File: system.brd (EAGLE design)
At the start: 160 x 100 mm, 131 parts, among them IC1 TPS7B8650BQDDARQ1, IC2 TLV9101IDBVR, IC3 TLV9101IDBVR, J1 TSW-104-07-F-S, J2 163-179PH-EX, J3 RS1-02-G, SW1 1825910-6, SW2 1825910-6, SW3 1825910-6, U1 ATMEGA328PB-AU, Y1 ABL-16.000MHZ-B2

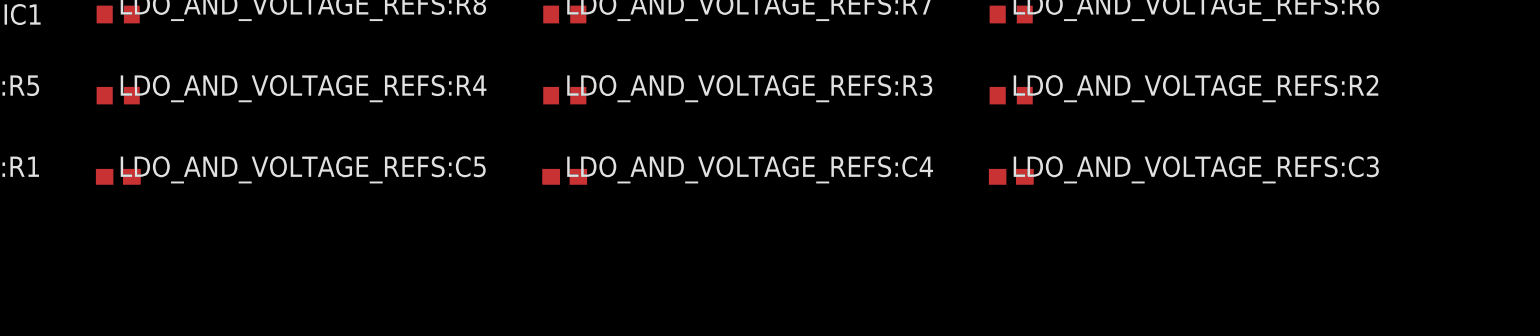
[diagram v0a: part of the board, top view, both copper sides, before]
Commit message: update some stuff
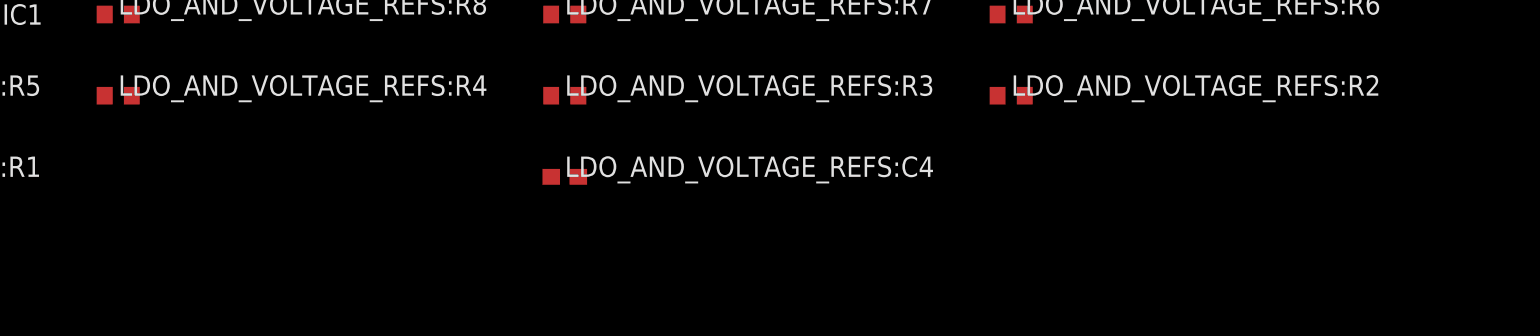
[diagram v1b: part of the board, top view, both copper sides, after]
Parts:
- removed LDO_AND_VOLTAGE_REFS:C3, LDO_AND_VOLTAGE_REFS:C5: 1uF, rcl:C0603
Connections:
- net 0: no longer LDO_AND_VOLTAGE_REFS:C3.2, LDO_AND_VOLTAGE_REFS:C5.2
- net VS_1.5V: no longer LDO_AND_VOLTAGE_REFS:C3.1
- net VS_2.5V: no longer LDO_AND_VOLTAGE_REFS:C5.1
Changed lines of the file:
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@@
 <attribute name="VALUE" x="-114.3" y="2.54" size="1.27" layer="27"/>
-</element>
-<element name="LDO_AND_VOLTAGE_REFS:C3" library="rcl" library_urn="urn:adsk.eagle:library:334" package="C0603" package3d_urn="urn:adsk.eagle:package:23616/2" value="1uF" x="-39.37" y="36.83" smashed="yes">
-<attribute name="NAME" x="-39.37" y="36.83" size="1.27" layer="25"/>
-<attribute name="POPULARITY" value="37" x="-39.37" y="36.83" size="1.778" layer="27" display="off"/>
-<attribute name="SPICEPREFIX" value="C" x="-39.37" y="36.83" size="1.778" layer="27" display="off"/>
-<attribute name="VALUE" x="-39.37" y="36.83" size="1.27" layer="27"/>
 </element>
 <element name="LDO_AND_VOLTAGE_REFS:C4" library="rcl" library_urn="urn:adsk.eagle:library:334" package="C0603" package3d_urn="urn:adsk.eagle:package:23616/2" value="1uF" x="-67.31" y="36.83" smashed="yes">
@@
 <attribute name="SPICEPREFIX" value="C" x="-67.31" y="36.83" size="1.778" layer="27" display="off"/>
 <attribute name="VALUE" x="-67.31" y="36.83" size="1.27" layer="27"/>
-</element>
-<element name="LDO_AND_VOLTAGE_REFS:C5" library="rcl" library_urn="urn:adsk.eagle:library:334" package="C0603" package3d_urn="urn:adsk.eagle:package:23616/2" value="1uF" x="-95.25" y="36.83" smashed="yes">
-<attribute name="NAME" x="-95.25" y="36.83" size="1.27" layer="25"/>
-<attribute name="POPULARITY" value="37" x="-95.25" y="36.83" size="1.778" layer="27" display="off"/>
-<attribute name="SPICEPREFIX" value="C" x="-95.25" y="36.83" size="1.778" layer="27" display="off"/>
-<attribute name="VALUE" x="-95.25" y="36.83" size="1.27" layer="27"/>
 </element>
 <element name="LDO_AND_VOLTAGE_REFS:IC1" library="TLV9101IDBVR" package="SOT95P280X145-5N" value="TLV9101IDBVR" x="-111.76" y="46.99" smashed="yes">
@@
 <contactref element="LDO_AND_VOLTAGE_REFS:IC3" pad="4"/>
 <contactref element="LDO_AND_VOLTAGE_REFS:IC3" pad="1"/>
-<contactref element="LDO_AND_VOLTAGE_REFS:C3" pad="1"/>
 <wire x1="-58.4" y1="53.02" x2="-104.99" y2="205.74" width="0" layer="19" extent="1-1"/>
 <wire x1="-55.9" y1="51.12" x2="-58.4" y2="53.02" width="0" layer="19" extent="1-1"/>
-<wire x1="-40.22" y1="36.83" x2="-55.9" y2="51.12" width="0" layer="19" extent="1-1"/>
 </signal>
 <signal name="VS_2.5V">
@@
 <contactref element="LDO_AND_VOLTAGE_REFS:IC2" pad="1"/>
 <contactref element="LDO_AND_VOLTAGE_REFS:IC2" pad="4"/>
-<contactref element="LDO_AND_VOLTAGE_REFS:C5" pad="1"/>
 <wire x1="-29.19" y1="53.02" x2="-49.11" y2="205.74" width="0" layer="19" extent="1-1"/>
 <wire x1="-26.69" y1="51.12" x2="-29.19" y2="53.02" width="0" layer="19" extent="1-1"/>
-<wire x1="-96.1" y1="36.83" x2="-29.19" y2="53.02" width="0" layer="19" extent="1-1"/>
 </signal>
 <signal name="ADC_EXT_INT">
@@
 <contactref element="BATTERY_AND_BUCK:C5" pad="2"/>
 <contactref element="BATTERY_AND_BUCK:C6" pad="2"/>
-<contactref element="LDO_AND_VOLTAGE_REFS:C5" pad="2"/>
 <contactref element="LDO_AND_VOLTAGE_REFS:IC3" pad="2"/>
 <contactref element="LDO_AND_VOLTAGE_REFS:IC1" pad="2"/>
@@
 <contactref element="LDO_AND_VOLTAGE_REFS:IC2" pad="2"/>
 <contactref element="LDO_AND_VOLTAGE_REFS:J1" pad="2"/>
-<contactref element="LDO_AND_VOLTAGE_REFS:C3" pad="2"/>
 <contactref element="LDO_AND_VOLTAGE_REFS:R6" pad="1"/>
 <contactref element="BANDGAP_REF:Q1" pad="5"/>
@@
 <wire x1="-40.22" y1="46.99" x2="-29.19" y2="52.07" width="0" layer="19" extent="1-1"/>
 <wire x1="-40.22" y1="41.91" x2="-40.22" y2="46.99" width="0" layer="19" extent="1-1"/>
-<wire x1="-38.52" y1="36.83" x2="-40.22" y2="41.91" width="0" layer="19" extent="1-1"/>
-<wire x1="-35.56" y1="20.32" x2="-38.52" y2="36.83" width="0" layer="19" extent="1-1"/>
 <wire x1="-58.4" y1="52.07" x2="-40.22" y2="46.99" width="0" layer="19" extent="1-1"/>
 <wire x1="-57.59" y1="68.18" x2="-58.4" y2="52.07" width="0" layer="19" extent="1-1"/>
 <wire x1="-49.09" y1="68.98" x2="-57.59" y2="68.18" width="0" layer="19" extent="1-1"/>
 <wire x1="-66.46" y1="36.83" x2="-58.4" y2="52.07" width="0" layer="19" extent="1-1"/>
+<wire x1="-35.56" y1="20.32" x2="-40.22" y2="41.91" width="0" layer="19" extent="1-1"/>
 <wire x1="-131.23" y1="102.87" x2="-107.1" y2="102.87" width="0" layer="19" extent="1-1"/>
 <wire x1="-132.93" y1="90.17" x2="-131.23" y2="102.87" width="0" layer="19" extent="1-1"/>
-<wire x1="-94.4" y1="36.83" x2="-66.46" y2="36.83" width="0" layer="19" extent="1-1"/>
-<wire x1="-96.1" y1="41.91" x2="-94.4" y2="36.83" width="0" layer="19" extent="1-1"/>
-<wire x1="-113.01" y1="46.99" x2="-96.1" y2="41.91" width="0" layer="19" extent="1-1"/>
 <wire x1="-99.48" y1="161.29" x2="-70.27" y2="161.29" width="0" layer="19" extent="1-1"/>
 <wire x1="-128.69" y1="161.29" x2="-99.48" y2="161.29" width="0" layer="19" extent="1-1"/>
-<wire x1="-85.51" y1="2.54" x2="-94.4" y2="36.83" width="0" layer="19" extent="1-1"/>
-<wire x1="-113.45" y1="2.54" x2="-85.51" y2="2.54" width="0" layer="19" extent="1-1"/>
-<wire x1="-132.93" y1="-10.16" x2="-113.45" y2="2.54" width="0" layer="19" extent="1-1"/>
-<wire x1="-132.93" y1="-13.97" x2="-132.93" y2="-10.16" width="0" layer="19" extent="1-1"/>
-<wire x1="-131.23" y1="-19.05" x2="-132.93" y2="-13.97" width="0" layer="19" extent="1-1"/>
-<wire x1="-131.23" y1="-24.13" x2="-131.23" y2="-19.05" width="0" layer="19" extent="1-1"/>
-<wire x1="-131.23" y1="-29.21" x2="-131.23" y2="-24.13" width="0" layer="19" extent="1-1"/>
+<wire x1="-96.1" y1="41.91" x2="-66.46" y2="36.83" width="0" layer="19" extent="1-1"/>
+<wire x1="-113.01" y1="46.99" x2="-96.1" y2="41.91" width="0" layer="19" extent="1-1"/>
 <wire x1="-101.18" y1="196.85" x2="-99.48" y2="161.29" width="0" layer="19" extent="1-1"/>
 <wire x1="-108.37" y1="205.74" x2="-101.18" y2="196.85" width="0" layer="19" extent="1-1"/>
@@
 <wire x1="-123.17" y1="210.82" x2="-123.61" y2="205.74" width="0" layer="19" extent="1-1"/>
 <wire x1="-114.72" y1="196.85" x2="-113.45" y2="205.74" width="0" layer="19" extent="1-1"/>
+<wire x1="-85.51" y1="2.54" x2="-66.46" y2="36.83" width="0" layer="19" extent="1-1"/>
+<wire x1="-113.45" y1="2.54" x2="-85.51" y2="2.54" width="0" layer="19" extent="1-1"/>
+<wire x1="-132.93" y1="-10.16" x2="-113.45" y2="2.54" width="0" layer="19" extent="1-1"/>
+<wire x1="-132.93" y1="-13.97" x2="-132.93" y2="-10.16" width="0" layer="19" extent="1-1"/>
+<wire x1="-131.23" y1="-19.05" x2="-132.93" y2="-13.97" width="0" layer="19" extent="1-1"/>
+<wire x1="-131.23" y1="-24.13" x2="-131.23" y2="-19.05" width="0" layer="19" extent="1-1"/>
+<wire x1="-131.23" y1="-29.21" x2="-131.23" y2="-24.13" width="0" layer="19" extent="1-1"/>
 <wire x1="116.86" y1="12.7" x2="-29.19" y2="52.07" width="0" layer="19" extent="1-1"/>
 <wire x1="122.77" y1="15.24" x2="116.86" y2="12.7" width="0" layer="19" extent="1-1"/>
